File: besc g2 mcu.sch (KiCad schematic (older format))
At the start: 36 parts, among them U7 SN74LVC1G04, U8 STM32F405RGTx, Y1 MCSJK-7I-8.00-18-10-60-B-10

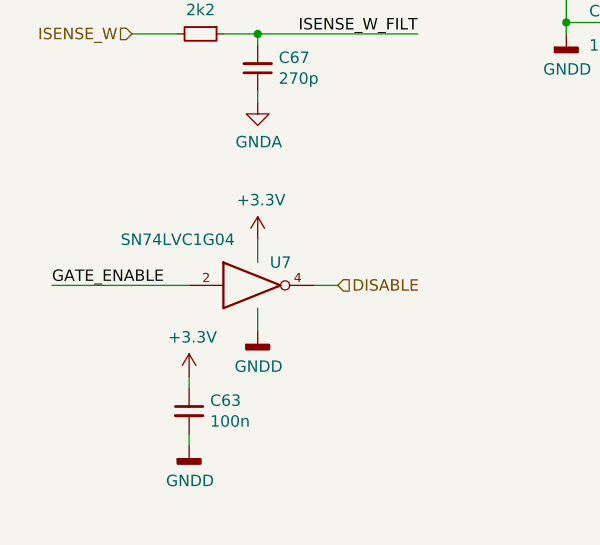
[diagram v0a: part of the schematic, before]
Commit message: u7 bug fixes
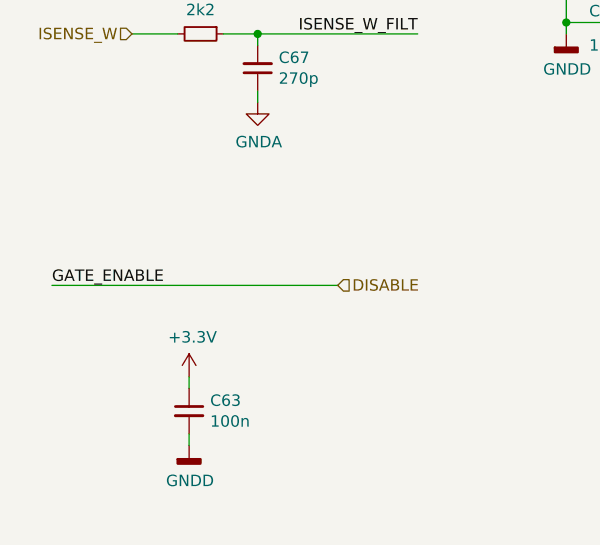
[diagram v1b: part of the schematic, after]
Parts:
- removed U7: SN74LVC1G04, Package_TO_SOT_SMD:SOT-23-5, symbol 74xGxx:74AHC1G04
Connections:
- net GATE_ENABLE is gone; now on net DISABLE: U8.57 (PB5)
- net GND renamed GNDD
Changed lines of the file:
@@
 	8250 1600 8250 1550
-$Comp
-L 74xGxx:74AHC1G04 U7
-U 1 1 5CEB8C8A
-P 2950 5050
-F 0 "U7" H 3050 5150 50  0000 C CNN
-F 1 "SN74LVC1G04" H 2600 5250 50  0000 C CNN
-F 2 "Package_TO_SOT_SMD:SOT-23-5" H 2950 5050 50  0001 C CNN
-F 3 "http://www.ti.com/lit/sg/scyt129e/scyt129e.pdf" H 2950 5050 50  0001 C CNN
-	1    2950 5050
-	1    0    0    -1
-$EndComp
-$Comp
-L power:GNDD #PWR084
-U 1 1 5CEB9CDA
-P 2950 5250
-F 0 "#PWR084" H 2950 5000 50  0001 C CNN
-F 1 "GNDD" H 2954 5095 50  0000 C CNN
-F 2 "" H 2950 5250 50  0001 C CNN
-F 3 "" H 2950 5250 50  0001 C CNN
-	1    2950 5250
-	1    0    0    -1
-$EndComp
-Wire Wire Line
-	2950 5150 2950 5250
-$Comp
-L power:+3.3V #PWR?
-U 1 1 5CEBBABE
-P 2950 4850
-AR Path="/5C9CD837/5CEBBABE" Ref="#PWR?"  Part="1"
-AR Path="/5CA11DF8/5CEBBABE" Ref="#PWR083"  Part="1"
-F 0 "#PWR083" H 2950 4700 50  0001 C CNN
-F 1 "+3.3V" H 2965 5023 50  0000 C CNN
-F 2 "" H 2950 4850 50  0001 C CNN
-F 3 "" H 2950 4850 50  0001 C CNN
-	1    2950 4850
-	1    0    0    -1
-$EndComp
-Wire Wire Line
-	2950 4950 2950 4850
 $Comp
 L Device:C_Small C63
@@
 Wire Wire Line
 	2650 5700 2650 5750
-Wire Wire Line
-	3200 5050 3300 5050
 $Comp
 L Device:C_Small C65
@@
 Text Label 2050 5050 0    50   ~ 0
 GATE_ENABLE
-Wire Wire Line
-	2650 5050 2050 5050
 Text HLabel 7100 4600 2    50   Input ~ 0
 RC_PWM
@@
 Wire Wire Line
 	2350 1600 2600 1600
+Wire Wire Line
+	2050 5050 3300 5050
 $EndSCHEMATC
